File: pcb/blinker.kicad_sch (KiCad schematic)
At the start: 15 parts, among them J1 ISP, U1 ATtiny10-TS

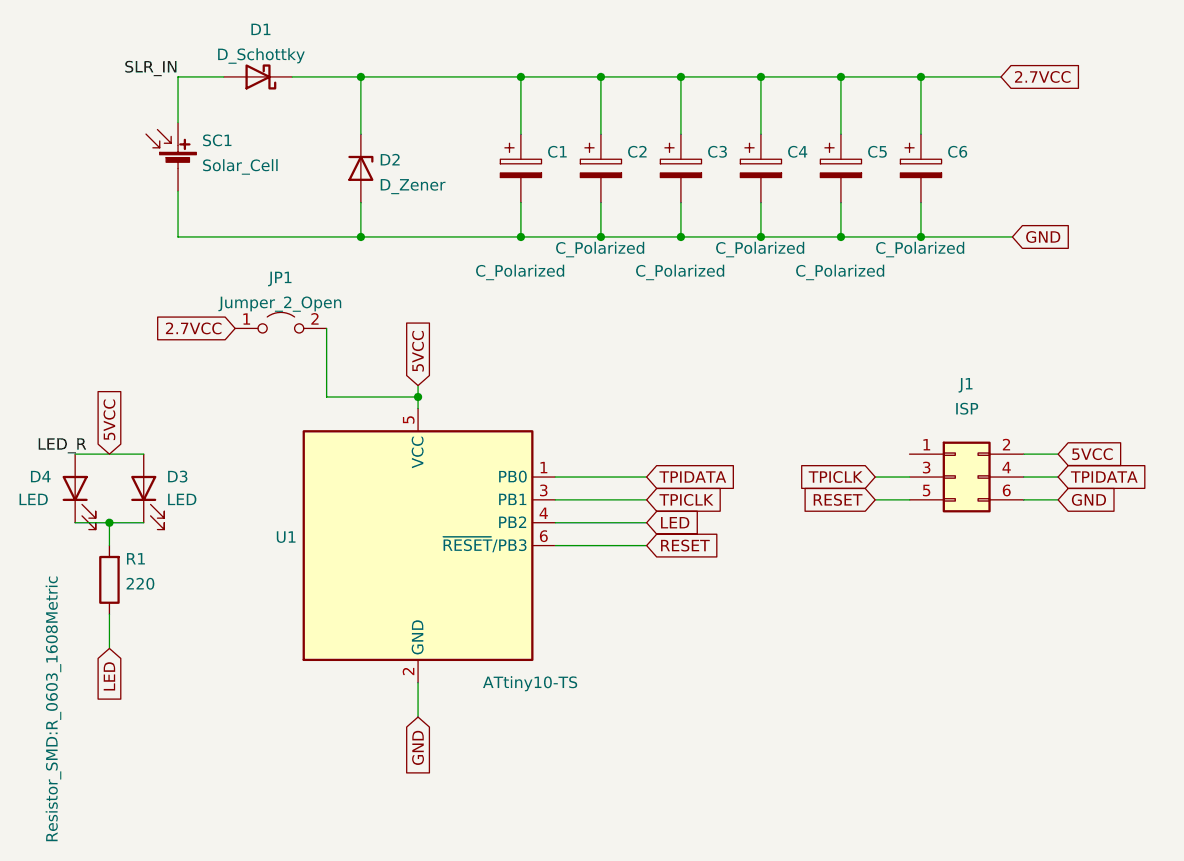
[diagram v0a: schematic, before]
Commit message: v1.2 of PCB
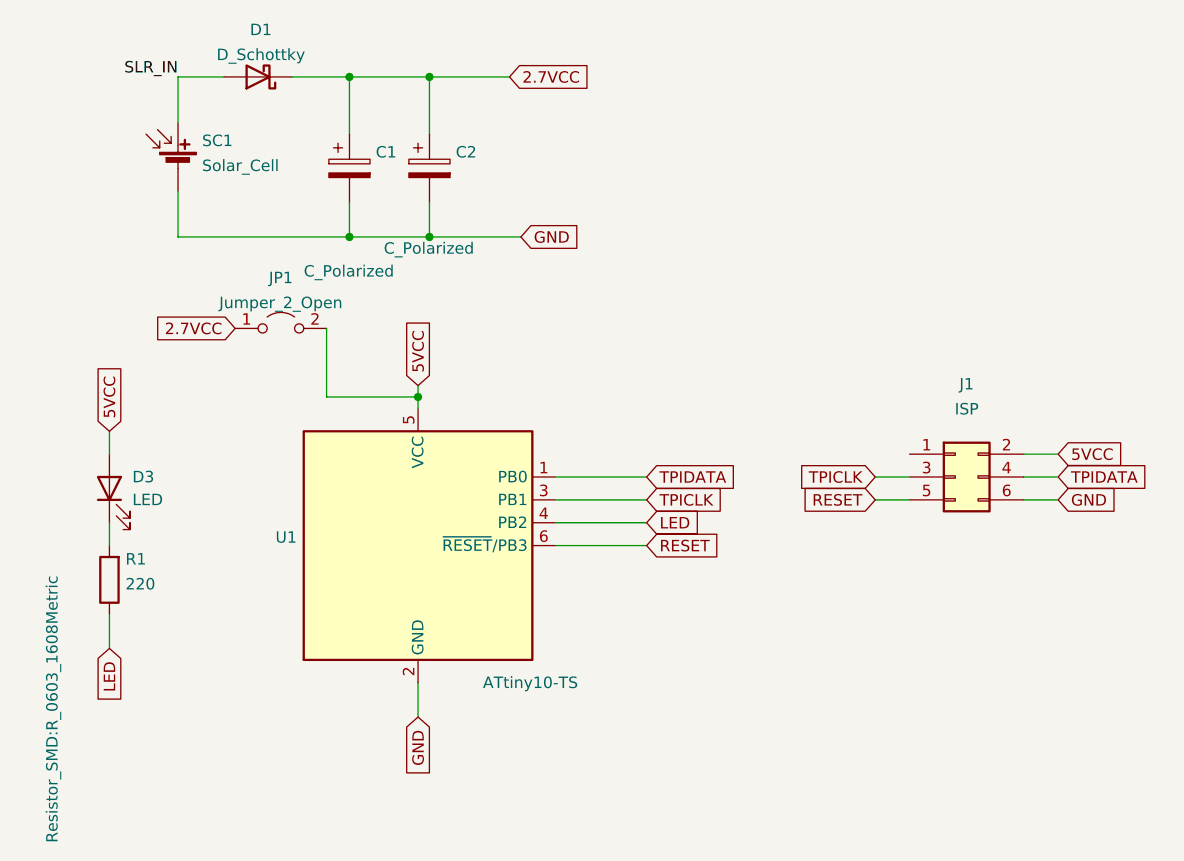
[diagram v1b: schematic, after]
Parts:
- removed C1, C2, C3, C4: C_Polarized, Capacitor_THT:CP_Radial_D16.0mm_P7.50mm, symbol Device:C_Polarized
- removed D2: D_Zener, Diode_SMD:D_SOD-123, symbol Device:D_Zener
- removed D4: LED, Connector_PinHeader_2.54mm:PinHeader_1x02_P2.54mm_Vertical, symbol Device:LED
- renumbered C5 to C1, C6 to C2
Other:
- moved on the sheet: C1, C2, D3
